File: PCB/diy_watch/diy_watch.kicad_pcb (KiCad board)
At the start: 2 copper layers, 37 x 37 mm, 34 parts, among them J1 Debug Port, P1 USB_C_Plug_USB2.0, SW1 SW_Push, U1 W25Q32JVSS, U2 DS3231MZ, U3 RP2040, U5 LTC4054ES5-4.2, Y1 12MHz_crystal

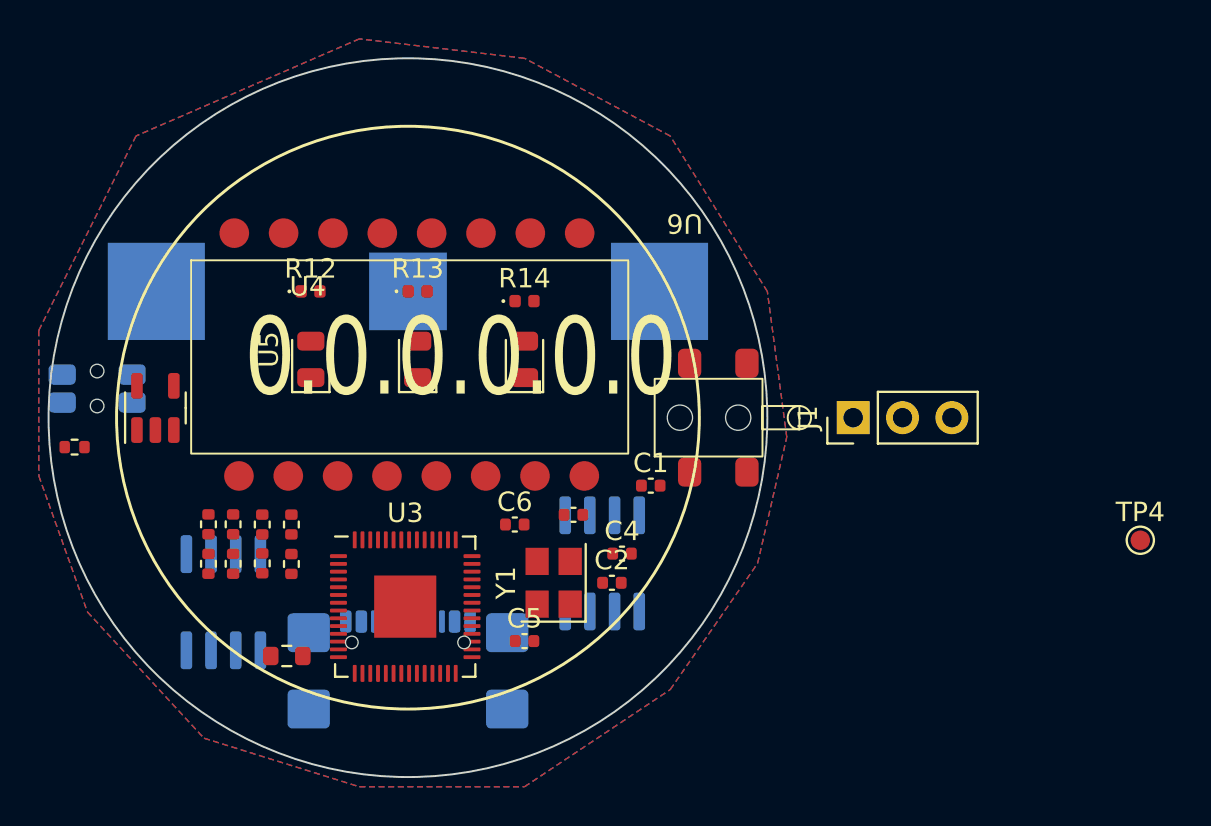
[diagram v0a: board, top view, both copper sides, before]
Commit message: Routed most of the PCB, big staggetti
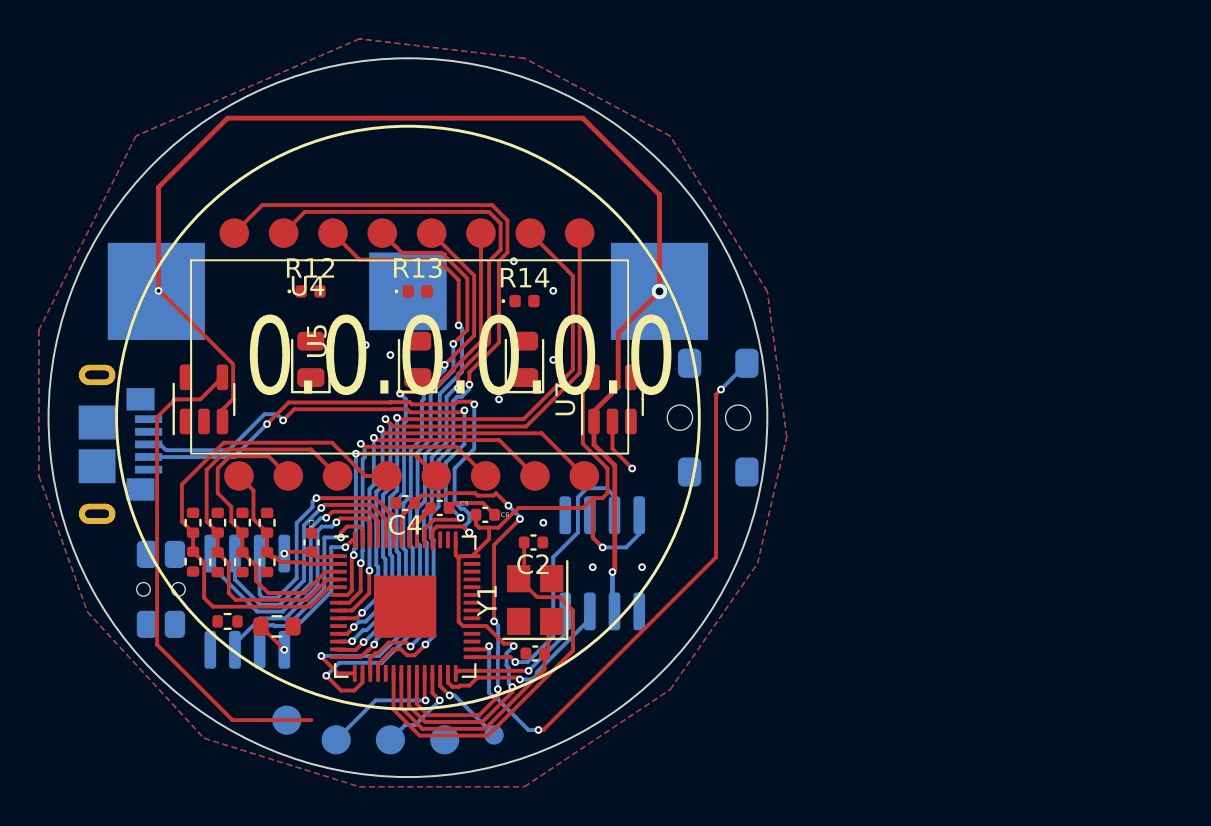
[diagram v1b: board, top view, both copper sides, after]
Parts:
- removed P1: USB_C_Plug_USB2.0, Connector_USB:USB_C_Receptacle_GCT_USB4110
- added TP1: TP_SWCLK, TestPoint:TestPoint_Pad_D1.5mm, B.Cu at (146.3, 116.6)
- added TP2: TP_GND, TestPoint:TestPoint_Pad_D1.5mm, B.Cu at (151.9, 116.6)
- added TP3: TP_SWD, TestPoint:TestPoint_Pad_D1.5mm, B.Cu at (149.1, 116.6)
- added TP5: TP_3V3, TestPoint:TestPoint_Pad_D1.5mm, B.Cu at (143.8, 115.6)
- added U7: XC6210B332MR, Package_TO_SOT_SMD:SOT-23-5, F.Cu at (160.5, 99.1)
- J1: value Debug Port -> USB_B_Micro; footprint Connector_PinHeader_2.54mm:PinHeader_1x03_P2.54mm_Vertical -> Connector_USB:USB_Micro-B_GCT_USB3076-30-A; moved to B.Cu
- TP4, U6: moved to B.Cu
- moved J1 37.7 mm to (135.2, 101.4)
- moved TP4 34.7 mm to (154.4, 116.3), turned to 180 degrees
- moved C1 17.7 mm to (145.0, 106.4), turned to 90 degrees
- moved R2 11.9 mm to (140.7, 110.5), turned to 180 degrees
- moved C4 11.5 mm to (149.9, 104.4), turned to 180 degrees
- moved SW1 10.8 mm to (137.3, 108.8), turned to 90 degrees
- moved C5 8.12 mm to (151.6, 104.6)
- moved C3 7.41 mm to (156.6, 112.1)
- moved C2 4.54 mm to (156.5, 106.4), turned to 180 degrees
- moved R7 3.79 mm to (140.2, 105.4)
- moved R8 3.79 mm to (140.2, 107.4)
- moved R10 3.56 mm to (138.9, 107.4)
- moved R9 3.56 mm to (138.9, 105.4)
- moved R3 3.02 mm to (142.7, 105.4)
- moved R4 3.02 mm to (142.7, 107.4)
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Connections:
- J1 pad 1: Net-(J1-Pin_1) -> +5V
- J1 pad 2: GND -> /usb_D-
- J1 pad 3: Net-(J1-Pin_3) -> /usb_D+
- R3 pad 1: +3V3 -> +3.3V
- R5 pad 1: +3V3 -> +3.3V
- R7 pad 1: +3V3 -> +3.3V
- R9 pad 1: +3V3 -> +3.3V
- U2 pad 4: +3V3 -> +3.3V
- U3 pad 24: Net-(J1-Pin_1) -> Net-(U3-SWCLK)
- U3 pad 25: Net-(J1-Pin_3) -> Net-(U3-SWD)
- U3 pad 31: unconnected-(U3-GPIO20-Pad31) -> /light_en
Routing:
- net +BATT: track 0.00 -> 66.2 mm, vias 0 -> 3
- net +3.3V: track 0.00 -> 50.4 mm, vias 0 -> 4
- net /L: track 0.00 -> 42.4 mm, vias 0 -> 2
- net /K: track 0.00 -> 39.1 mm, vias 0 -> 2
- net /J: track 0.00 -> 35.0 mm, vias 0 -> 2
- net /I: track 0.00 -> 31.9 mm, vias 0 -> 2
- net /F: track 0.00 -> 31.5 mm, vias 0 -> 2
- net /E: track 0.00 -> 31.3 mm, vias 0 -> 2
- net /light_sw: track 0.00 -> 30.2 mm, vias 0 -> 3
- net /usb_D-: track 0.00 -> 28.9 mm, vias 0 -> 4
- net /usb_D+: track 0.00 -> 26.5 mm, vias 0 -> 3
- net /H: track 0.00 -> 26.4 mm, vias 0 -> 2
- net /G: track 0.00 -> 26.3 mm, vias 0 -> 2
- net /COM4: track 0.00 -> 26.0 mm
- net +5V: track 0.00 -> 25.7 mm
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- added copper zone on B.Cu, net GND
- added copper zone on F.Cu, net GND
- removed copper zone on B.Cu, net (none)
- removed copper zone on F.Cu, net (none)
